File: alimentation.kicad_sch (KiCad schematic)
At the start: 15 parts, among them J3 Conn_01x02, J4 Conn_01x02, J5 Conn_01x02

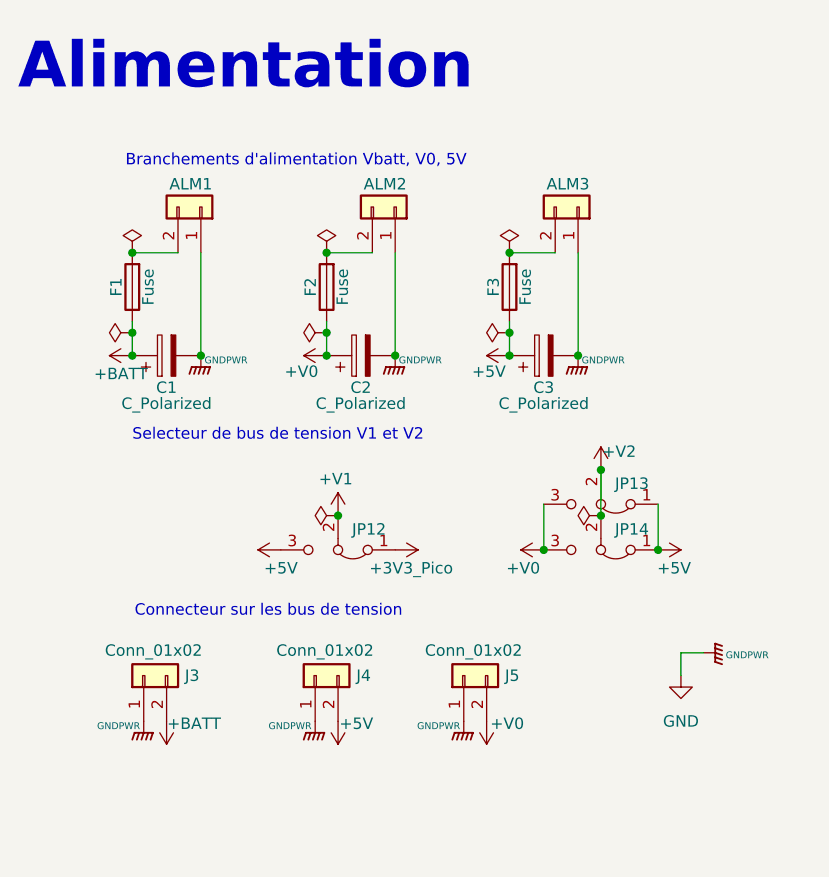
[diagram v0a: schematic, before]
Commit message: placement des empreintes début
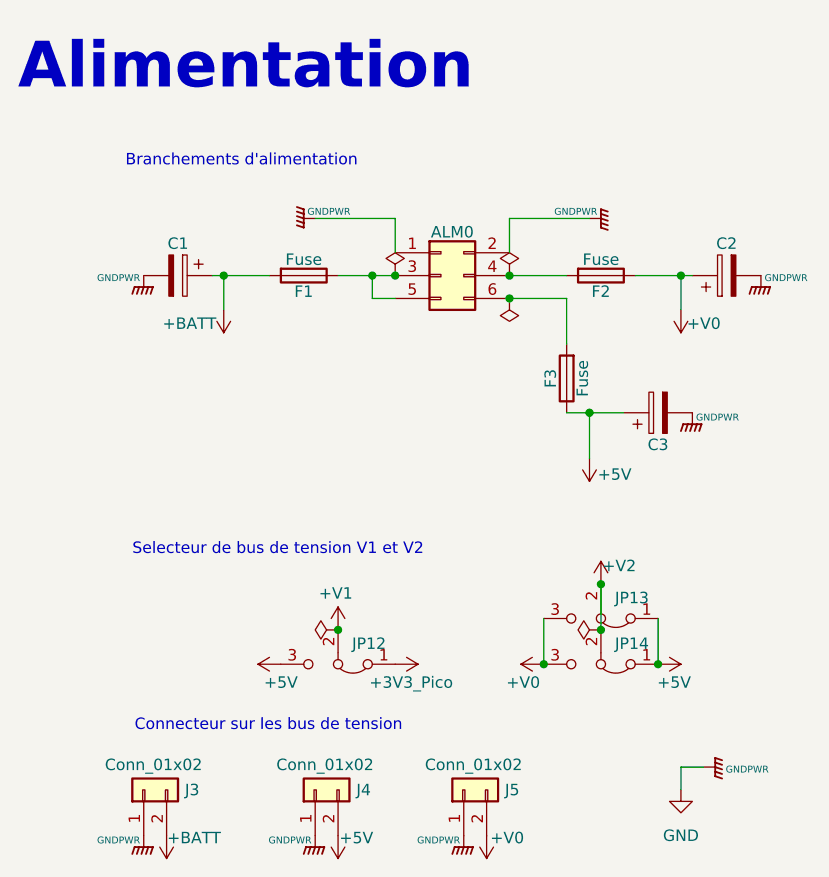
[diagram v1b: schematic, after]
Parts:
- removed ALM1, ALM2, ALM3: Conn_01x02, Connector_AMASS:AMASS_XT30PW-F_1x02_P2.50mm_Horizontal, symbol Connector_Generic:Conn_01x02
- added ALM0: Conn_02x03_Odd_Even, Connector_Molex:Molex_Mini-Fit_Jr_5569-06A2_2x03_P4.20mm_Horizontal, symbol Connector_Generic:Conn_02x03_Odd_Even
- J3, J4, J5: footprint Connector_PinHeader_2.54mm:PinHeader_1x02_P2.54mm_Vertical -> Connector_JST:JST_XH_B2B-XH-A_1x02_P2.50mm_Vertical
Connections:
- net +BATT: now also F1.2; no longer F1.1
- net GND: now also ALM0.1 (Pin_1), ALM0.2 (Pin_2)
- net at F2.2: now also ALM0.4 (Pin_4)
- net at F3.2: now also ALM0.6 (Pin_6)
- new net: ALM0.3 (Pin_3), ALM0.5 (Pin_5), F1.1
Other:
- note added: "Branchements d'alimentation"
- note removed: "Branchements d'alimentation Vbatt, V0, 5V"
- moved on the sheet: C1, C3, F2, F3, J3, J4, J5, JP12, JP13, JP14
